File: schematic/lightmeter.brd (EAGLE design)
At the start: 27.9 x 52.6 mm, 80 parts, among them IC2 MCP73831/OT, J1 AVR_SPI_PRG_6NS, Q1 NCHANNELMOSFET, Q10 PCHANNELMOSFET, Q11 NCHANNELMOSFET, Q12 NCHANNELMOSFET, Q13 NCHANNELMOSFET, Q14 NCHANNELMOSFET, Q16 NCHANNELMOSFET, Q2 PCHANNELMOSFET, Q3 NCHANNELMOSFET, Q4 PCHANNELMOSFET, Q5 NCHANNELMOSFET, Q6 PCHANNELMOSFET, Q7 NCHANNELMOSFET, Q8 PCHANNELMOSFET, Q9 PCHANNELMOSFET

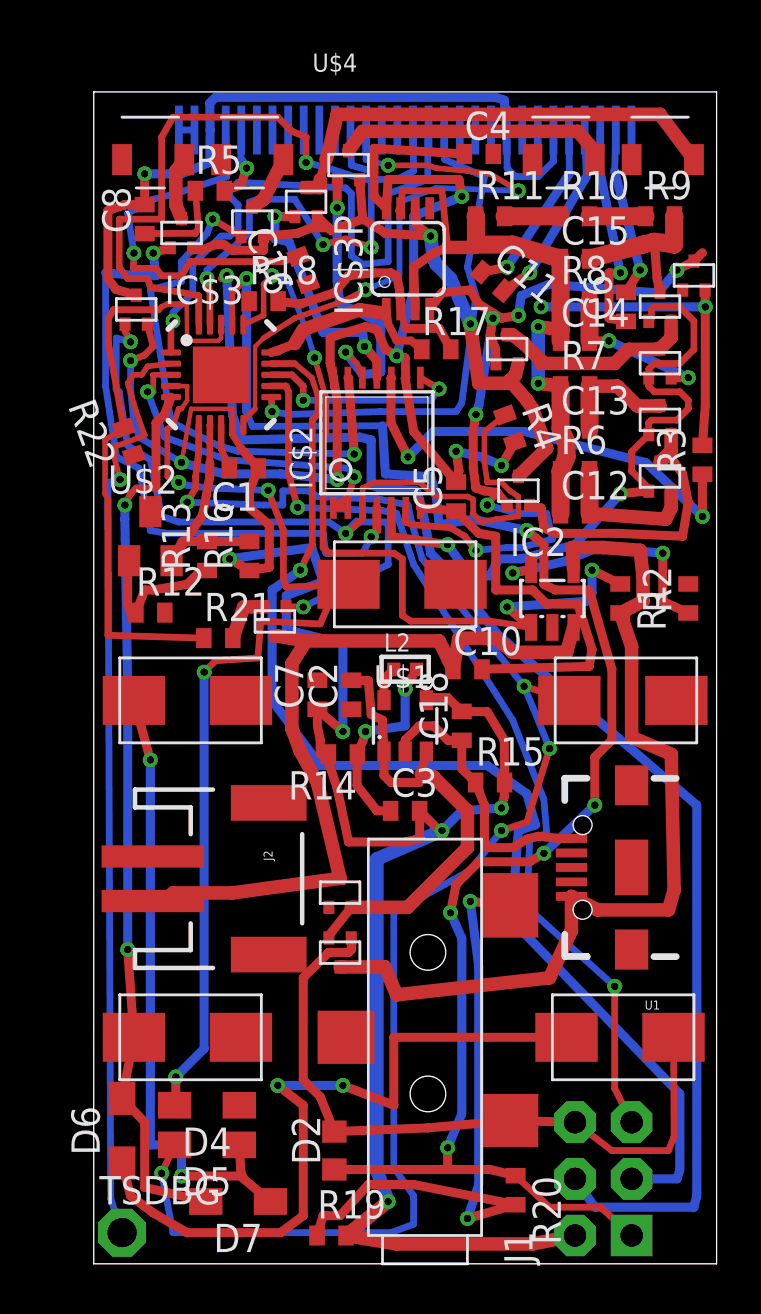
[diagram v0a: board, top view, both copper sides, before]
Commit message: More work on layout.
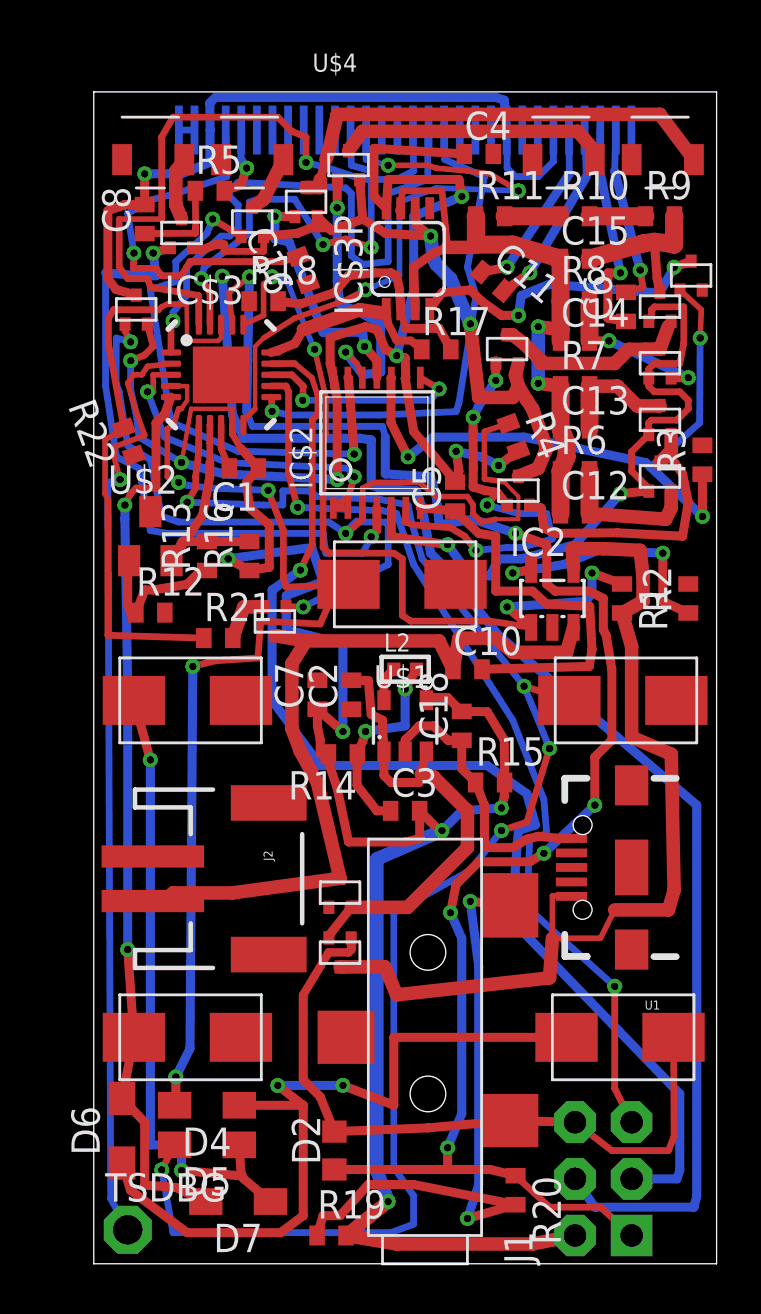
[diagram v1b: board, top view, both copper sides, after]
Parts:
- moved R4 0.41 mm to (17.6, 37.1)
- moved TSDBG 0.28 mm to (0.25, 1.52)
- moved Q7 0.13 mm to (25.5, 44.6)
- moved R1 0.08 mm to (22.4, 29.8)
- moved C5 0.05 mm to (14.9, 34.4)
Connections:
- net OAPWR: now also Q7.P$1
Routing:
- net GND: track 83.3 -> 69.1 mm, vias 2 -> 0
- net OAPWR: track 20.4 -> 29.6 mm, vias 2 -> 3
- net STG$2: track 23.9 -> 20.2 mm
- net N$8: track 32.6 -> 35.3 mm
- net N$26: track 30.6 -> 32.1 mm
- net N$6: track 14.7 -> 14.0 mm
- net PBI$2: track 40.0 -> 39.3 mm
- net AVRMISO/FLASHSYNC: track 75.3 -> 75.8 mm

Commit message: More work on layout.
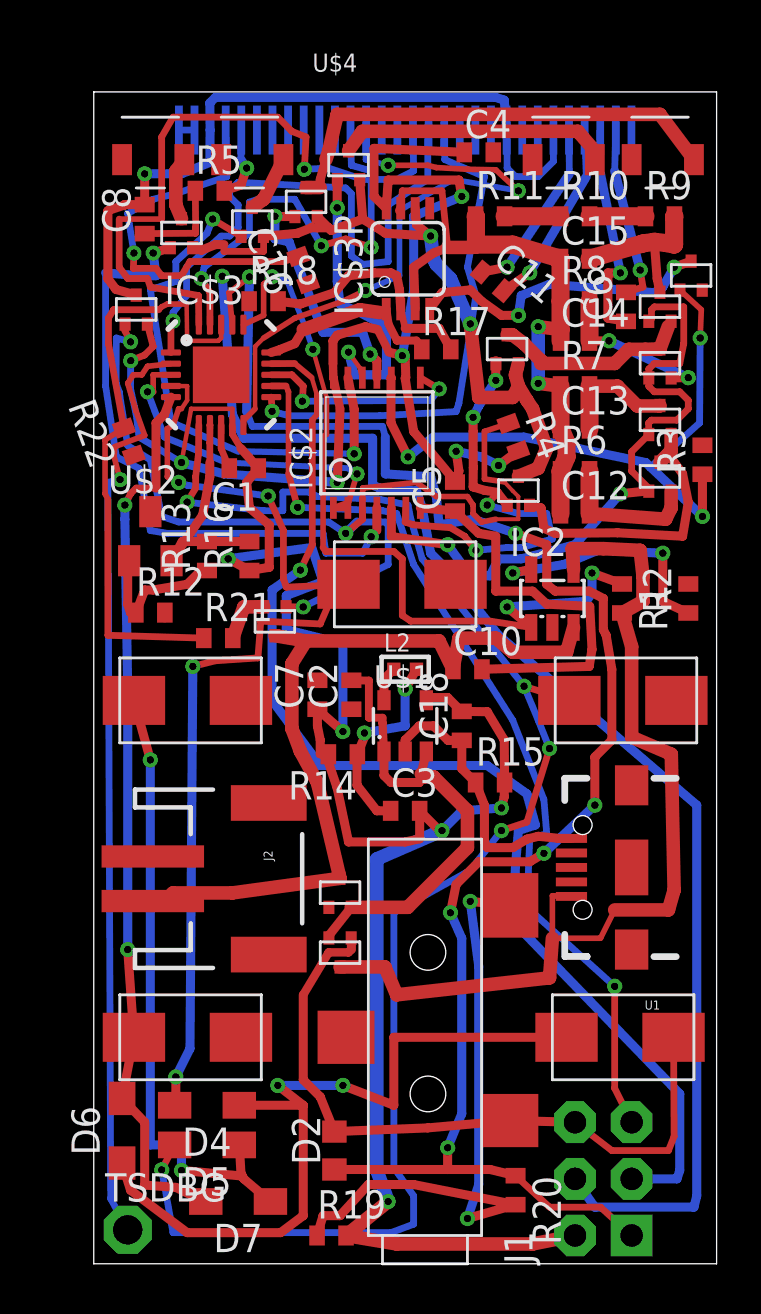
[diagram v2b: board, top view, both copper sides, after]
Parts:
- moved C4 0.07 mm to (16.0, 49.9)
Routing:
- net DIODESW$3: track 13.3 -> 13.9 mm

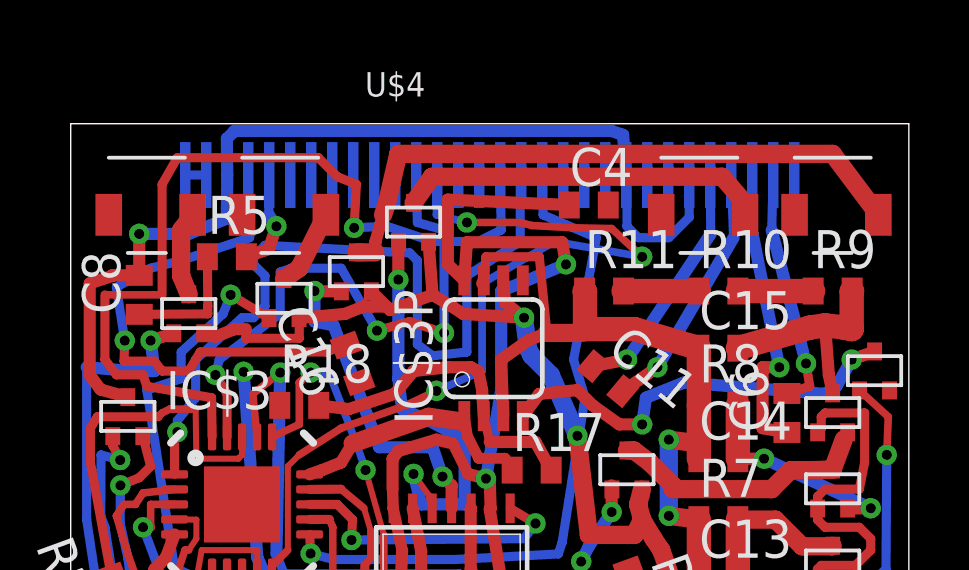
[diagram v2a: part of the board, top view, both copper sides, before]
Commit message: More work on layout.
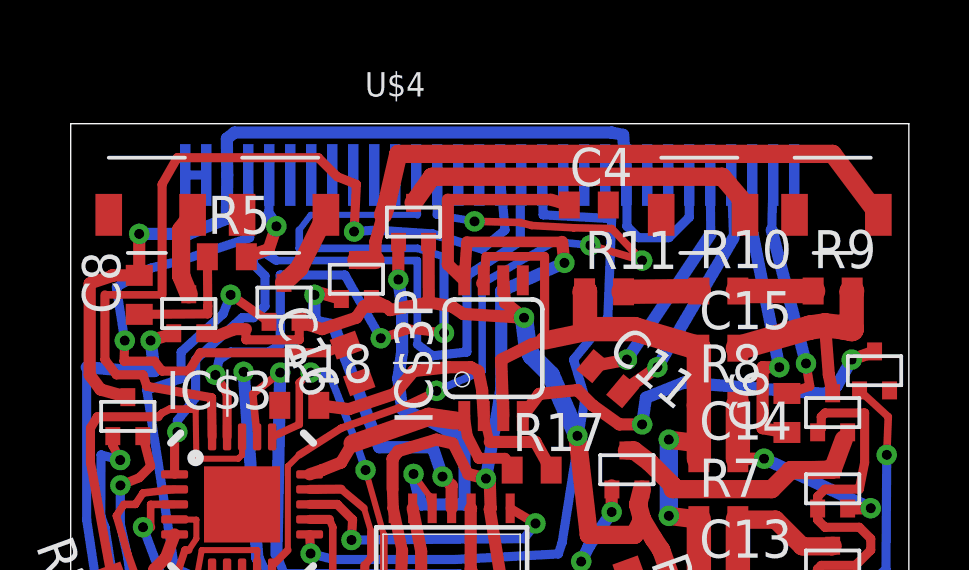
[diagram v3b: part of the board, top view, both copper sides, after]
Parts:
- moved Q14 0.25 mm to (8.26, 47.6)
- moved Q12 0.13 mm to (5.84, 46.9)
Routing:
- net SCRDAT: track 19.4 -> 27.5 mm
- net SCRCS: track 22.9 -> 24.3 mm
- net SCRCLK: track 28.3 -> 28.4 mm, vias 3 -> 4
